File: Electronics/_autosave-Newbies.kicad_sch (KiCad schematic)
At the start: 40 parts, among them J1 USB_C_Receptacle_USB2.0_14P, J2 Screw_Terminal_01x04, J3 Screw_Terminal_01x04, SW1 SW_Push, SW2 SW_Push, SW3 SW_Push, SW4 SW_Push, SW5 SW_Push, SW6 SW_Push, U1 ESP32-S3-WROOM-1, U2 NCP1117-3.3_SOT223, U3 NCP1117-3.3_SOT223, U4 MOTOR_L, U4 MOTOR_R

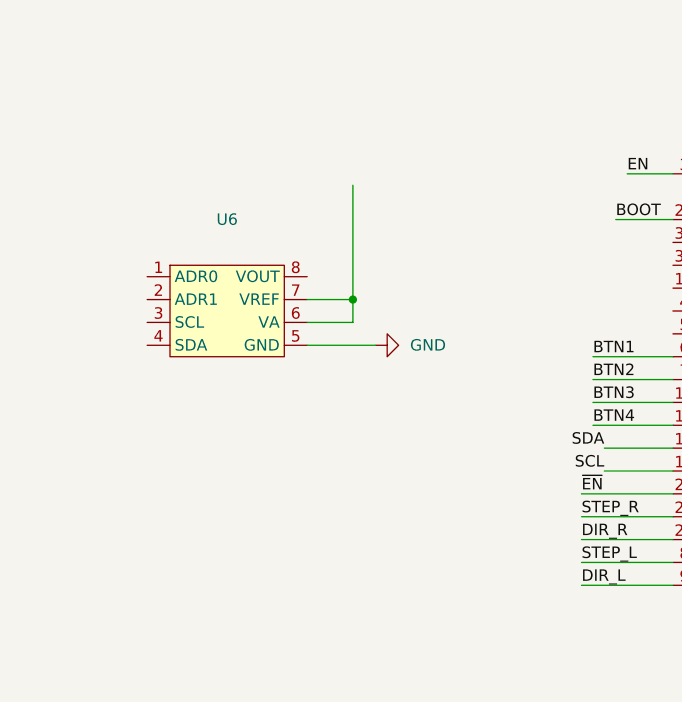
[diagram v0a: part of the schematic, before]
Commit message: trevor
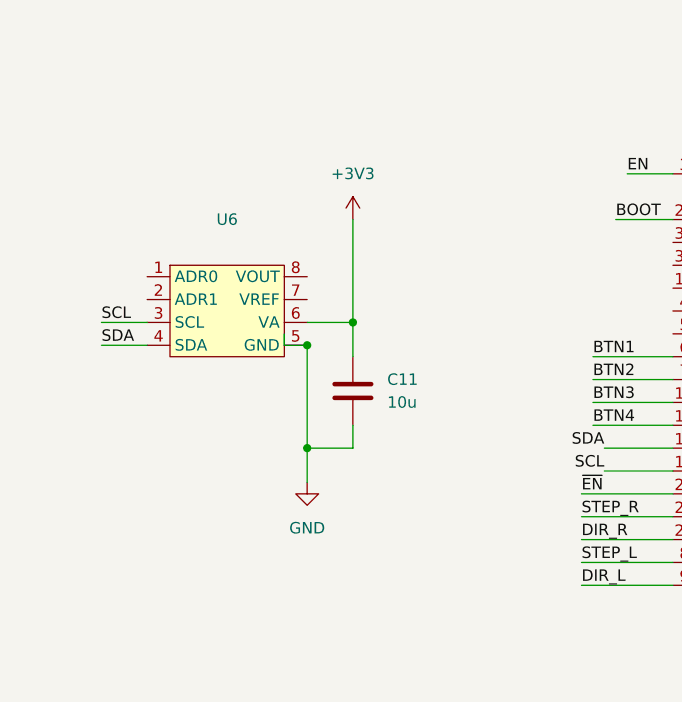
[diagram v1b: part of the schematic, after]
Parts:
- added C11: 10u, symbol Device:C
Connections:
- net +3V3: now also U6.6 (VA), C11.1
- net GND: now also C11.2
- net SCL: now also U6.3 (SCL)
- net SDA: now also U6.4 (SDA)
- net at U6.7 (VREF): no longer U6.6 (VA)
